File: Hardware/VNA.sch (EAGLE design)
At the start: 499 parts, among them IC1 ADL5801, IC10 LT5560, IC11 THS4521IDGKR, IC12 MCP33131D-10-E/MS, IC13 SI5351C, IC14 MAX2871, IC15 NCP702-3.3, IC16 RFSW6042, IC17 AP2114H, IC18 RFSW6042, IC19 MAX2871, IC2 LT5560, IC20 NCP702-3.3, IC21 AP2114H, IC22 QPC6324, IC23 RFSA3714, IC24 TRF37A73, IC25 QPC6324, IC26 QPC6324, IC27 QPC6324, IC28 LDL212PU50R, IC29 LDL212PU50R, IC3 THS4521IDGKR, IC30 LDL212PU50R, IC31 LDL212PU50R, IC32 TPS65265, IC34 NCP702-1.8, IC35 NCP702-1.8, IC36 NCP702-1.8, IC37 ADL5801, IC4 MCP33131D-10-E/MS, IC5 ADL5801, IC6 LT5560, IC7 THS4521IDGKR, IC8 MCP33131D-10-E/MS, IC9 STM32G431KB, J1 AMPHENOL_132289, J2 AMPHENOL_132289, J3 DCJ0202, J4 TYPE-C16P(073), Q1 FA-128 26MHz, T1 B012-617DB-1-63-B331, T2 B012-617DB-1-63-B331, T3 B012-617DB-1-63-B331, U2 6SLX9TQG144, U4 W25Q16BVSN, X4 DNP, X5 10MHz out, X6 10MHz in

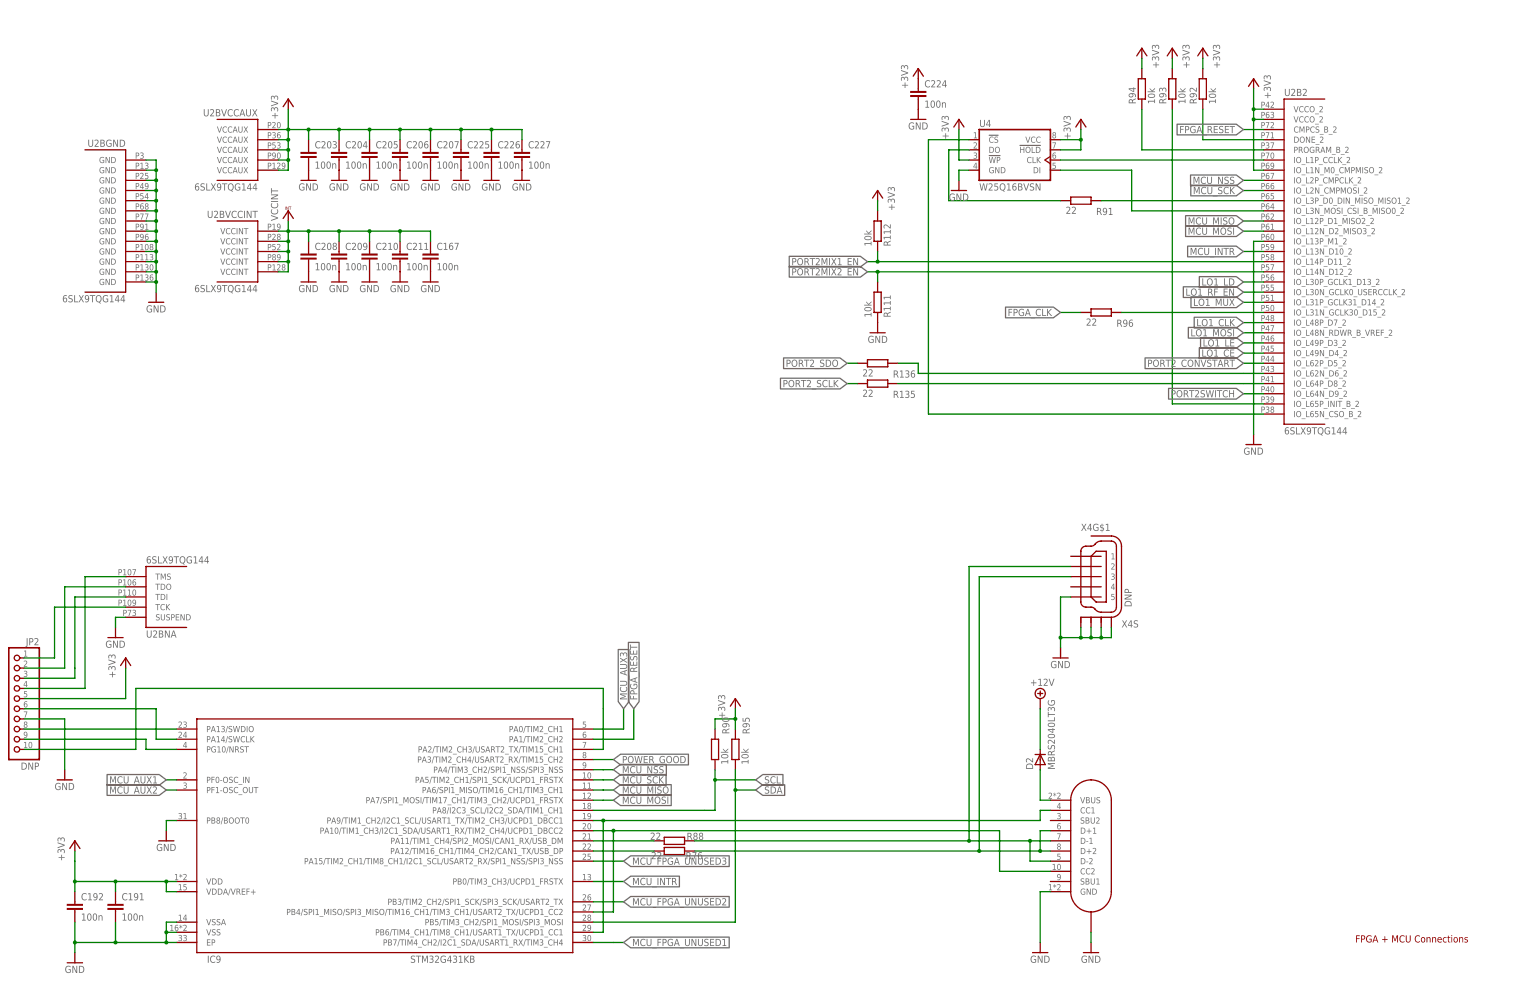
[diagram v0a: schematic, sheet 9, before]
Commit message: Routing completed
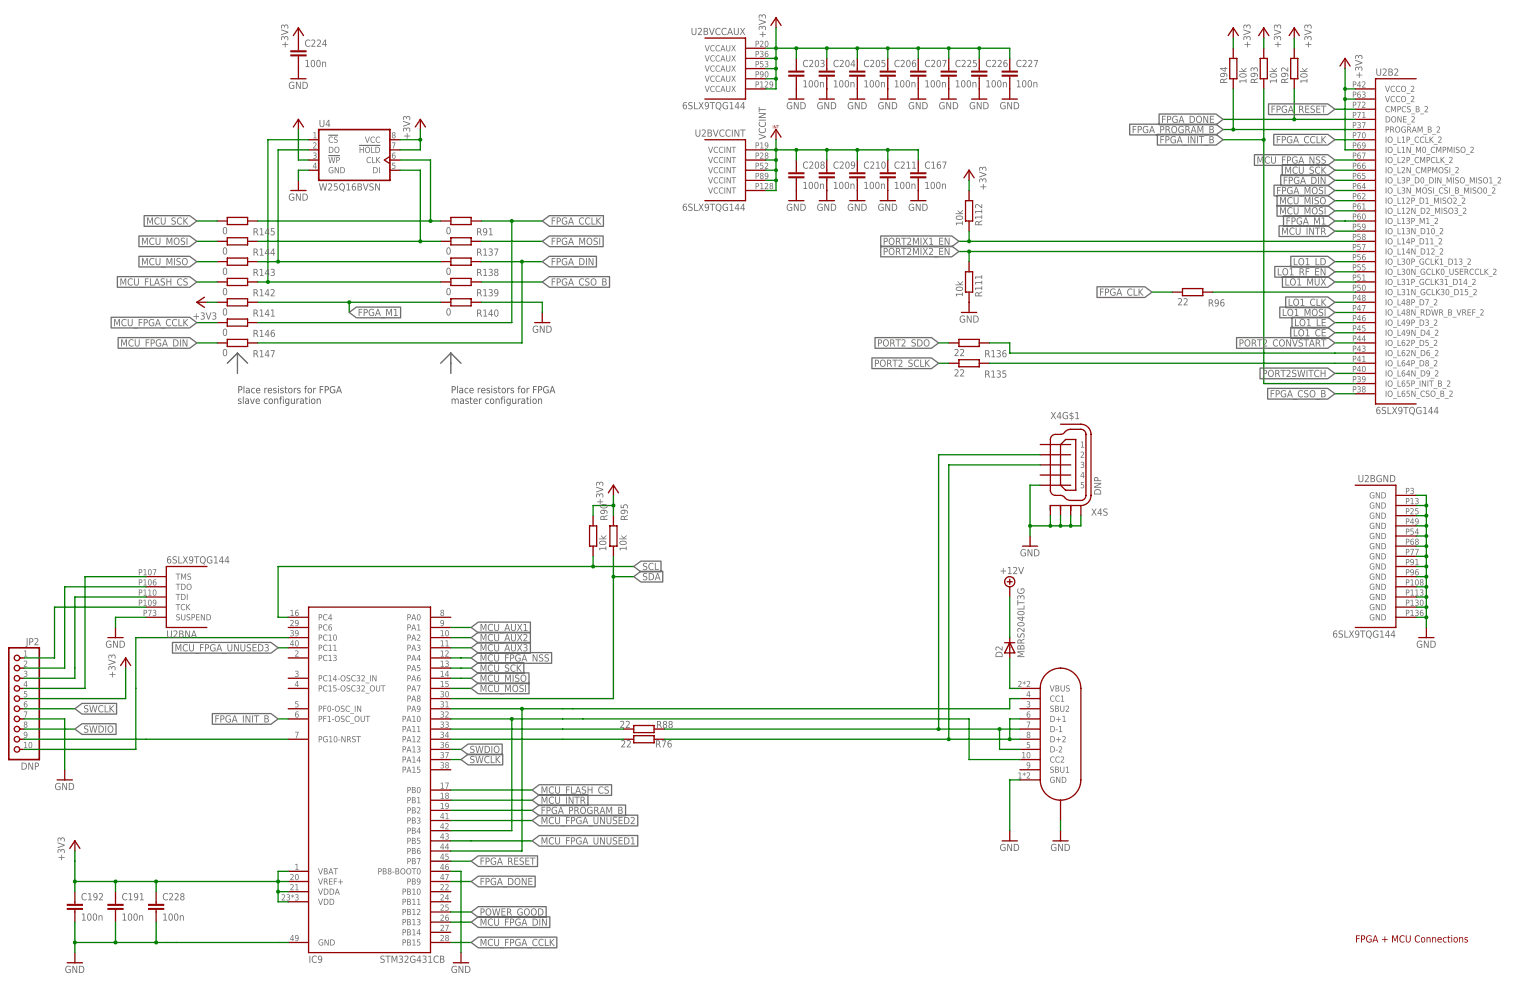
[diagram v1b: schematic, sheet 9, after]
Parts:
- added C228: 100n, rcl:C-EUC0402
- added R137, R138, R139, R140, R141, R142, R143, R144, R145, R146, R147: 0, rcl:R-EU_R0402
- IC9: value STM32G431KB -> STM32G431CB; device custom-ic:STM32G431KB -> custom-ic:STM32G431CB
- R91: value 22 -> 0
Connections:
- removed net FLACH_MOSI: U2B2.IO_L3N_MOSI_CSI_B_MISO0_2, U4.DI
- removed net FLASH_CLK: U2B2.IO_L1P_CCLK_2, U4.CLK
- removed net FLASH_CS: U2B2.IO_L65N_CSO_B_2, U4.!CS!
- removed net FLASH_MISO: R91.1, U4.DO
- removed net MCU_NSS: IC9.PA4/TIM3_CH2/SPI1_NSS/SPI3_NSS, U2B2.IO_L2P_CMPCLK_2
- removed net N$190: IC9.PA14/SWCLK, JP2.6
- removed net N$191: IC9.PA13/SWDIO, JP2.8
- removed net N$194: R92.1, U2B2.DONE_2
- removed net N$195: R93.1, U2B2.IO_L65P_INIT_B_2
- removed net N$196: R94.1, U2B2.PROGRAM_B_2
- new net FPGA_CCLK: R146.2, R91.2, U2B2.IO_L1P_CCLK_2
- new net FPGA_CSO_B: R139.2, U2B2.IO_L65N_CSO_B_2
- new net FPGA_DIN: R138.2, R147.2, U2B2.IO_L3P_D0_DIN_MISO_MISO1_2
- new net FPGA_DONE: IC9.PB9, R92.1, U2B2.DONE_2
- new net FPGA_INIT_B: IC9.PF1-OSC_OUT, R93.1, U2B2.IO_L65P_INIT_B_2
- new net FPGA_M1: R140.1, R141.2, U2B2.IO_L13P_M1_2
- new net FPGA_MOSI: R137.2, U2B2.IO_L3N_MOSI_CSI_B_MISO0_2
- new net FPGA_PROGRAM_B: IC9.PB2, R94.1, U2B2.PROGRAM_B_2
- new net MCU_FLASH_CS: IC9.PB0, R142.1
- new net MCU_FPGA_CCLK: IC9.PB15, R146.1
- new net MCU_FPGA_DIN: IC9.PB13, R147.1
- new net MCU_FPGA_NSS: IC9.PA4, U2B2.IO_L2P_CMPCLK_2
- new net N$237: R137.1, R144.2, U4.DI
- new net N$240: R138.1, R143.2, U4.DO
- new net N$241: R139.1, R142.2, U4.!CS!
- new net SWCLK: IC9.PA14, JP2.6
- new net SWDIO: IC9.PA13, JP2.8
- net +3V3: now also C228.1, IC9.VBAT, IC9.VDDA, IC9.VREF+, R141.1; no longer IC9.VDDA/VREF+
- net FPGA_RESET: now also IC9.PB7; no longer IC9.PA1/TIM2_CH2
- net GND: now also C228.2, IC9.GND, IC9.PB8-BOOT0, R140.2; no longer IC9.EP, IC9.PB8/BOOT0, IC9.VSS, IC9.VSSA, U2B2.IO_L13P_M1_2
- net MCU_AUX1: now also IC9.PA1; no longer IC9.PF0-OSC_IN
- net MCU_AUX2: now also IC9.PA2; no longer IC9.PF1-OSC_OUT
- net MCU_AUX3: now also IC9.PA3; no longer IC9.PA0/TIM2_CH1
- net MCU_FPGA_UNUSED1: now also IC9.PB5; no longer IC9.PB7/TIM4_CH2/I2C1_SDA/USART1_RX/TIM3_CH4
- net MCU_FPGA_UNUSED2: now also IC9.PB3; no longer IC9.PB3/TIM2_CH2/SPI1_SCK/SPI3_SCK/USART2_TX
- net MCU_FPGA_UNUSED3: now also IC9.PC11; no longer IC9.PA15/TIM2_CH1/TIM8_CH1/I2C1_SCL/USART2_RX/SPI1_NSS/SPI3_NSS
- net MCU_INTR: now also IC9.PB1; no longer IC9.PB0/TIM3_CH3/UCPD1_FRSTX
- net MCU_MISO: now also IC9.PA6, R143.1; no longer IC9.PA6/SPI1_MISO/TIM16_CH1/TIM3_CH1
- net MCU_MOSI: now also IC9.PA7, R144.1; no longer IC9.PA7/SPI1_MOSI/TIM17_CH1/TIM3_CH2/UCPD1_FRSTX
- net MCU_SCK: now also IC9.PA5, R145.1; no longer IC9.PA5/TIM2_CH1/SPI1_SCK/UCPD1_FRSTX
- net N$187: now also IC9.PA11; no longer IC9.PA11/TIM1_CH4/SPI2_MOSI/CAN1_RX/USB_DM
- net N$188: now also IC9.PA12; no longer IC9.PA12/TIM16_CH1/TIM4_CH2/CAN1_TX/USB_DP
- net N$192: now also IC9.PG10-NRST; no longer IC9.PG10/NRST
- net N$193: now also IC9.PC10; no longer IC9.PA2/TIM2_CH3/USART2_TX/TIM15_CH1
- net N$197: now also R145.2, R91.1, U4.CLK; no longer R91.2, U2B2.IO_L3P_D0_DIN_MISO_MISO1_2
- net N$233: now also IC9.PA9, IC9.PB6; no longer IC9.PA9/TIM1_CH2/I2C1_SCL/USART1_TX/TIM2_CH3/UCPD1_DBCC1, IC9.PB6/TIM4_CH1/TIM8_CH1/USART1_TX/UCPD1_CC1
- net N$234: now also IC9.PA10, IC9.PB4; no longer IC9.PA10/TIM1_CH3/I2C1_SDA/USART1_RX/TIM2_CH4/UCPD1_DBCC2, IC9.PB4/SPI1_MISO/SPI3_MISO/TIM16_CH1/TIM3_CH1/USART2_TX/UCPD1_CC2
- net POWER_GOOD: now also IC9.PB12; no longer IC9.PA3/TIM2_CH4/USART2_RX/TIM15_CH2
- net SCL: now also IC9.PC4; no longer IC9.PA8/I2C3_SCL/I2C2_SDA/TIM1_CH1
- net SDA: now also IC9.PA8; no longer IC9.PB5/TIM3_CH2/SPI1_MOSI/SPI3_MOSI
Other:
- note added: "Place resistors for FPGA master configuration"
- note added: "Place resistors for FPGA slave configuration"
- moved on the sheet: C167, C203, C204, C205, C206, C207, C208, C209, C210, C211, C224, C225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
